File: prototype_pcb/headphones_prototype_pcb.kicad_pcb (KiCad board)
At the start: 2 copper layers, 59.8 x 62.2 mm, 52 parts, among them J1 LIGHTING_JACK, J2 CONN_01X10, J3 BOTTOM_FLEX_LIGHTNING, J4 CONN_01X10, J5 LIGHTNING_HEADPHONE_ADAPTER, J6 CONN_01X10, J7 IPHONE_HEADPHONE_JACK, J8 CONN_01X02, U1 SN74LVC1G123, U2 ADG774A, U3 SN74LVC1G123, U4 NC7S32

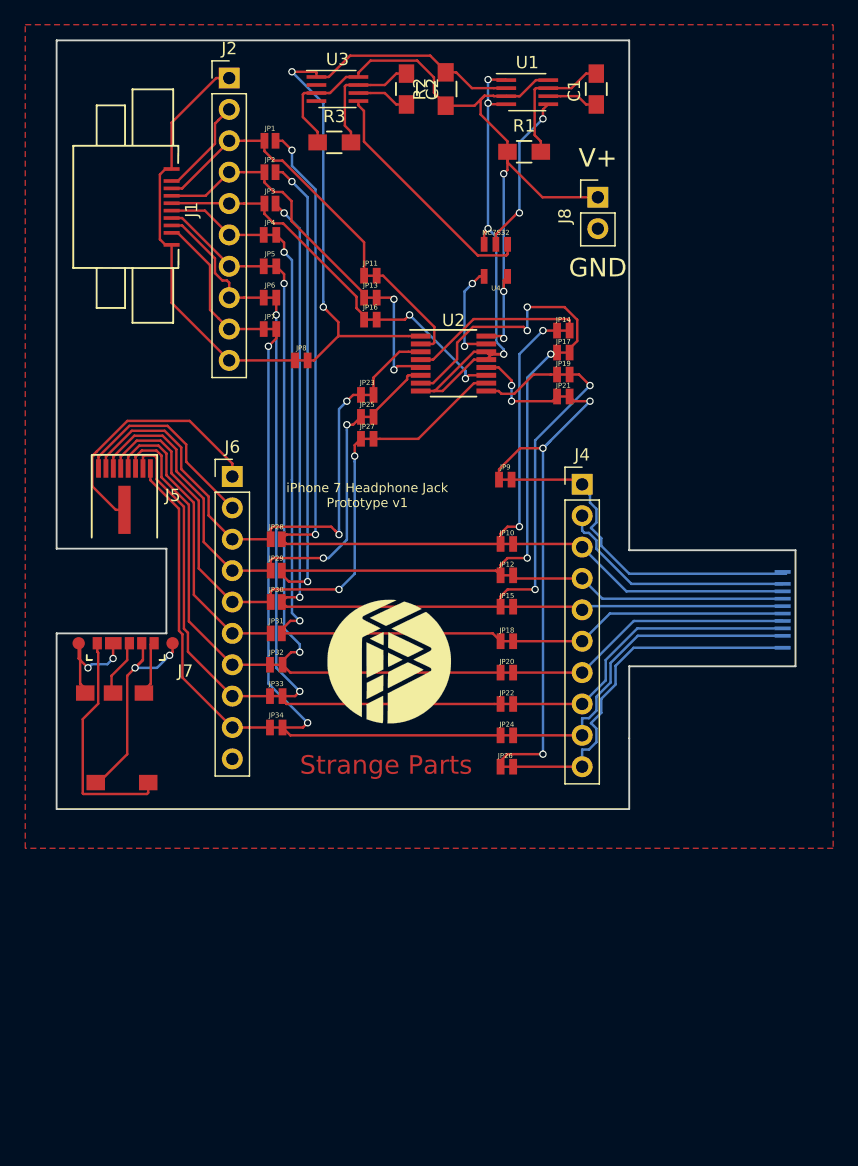
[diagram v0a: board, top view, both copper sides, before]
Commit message: Rigid prototype pcb v1.2
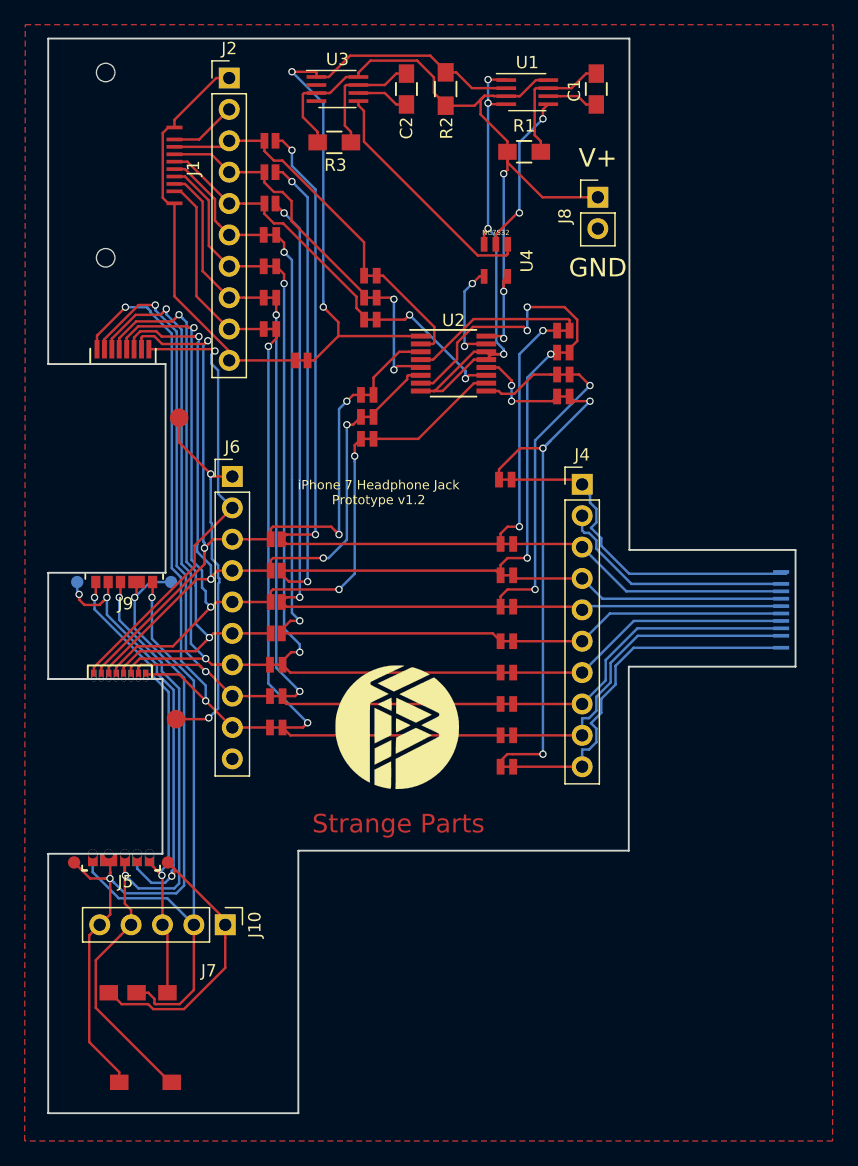
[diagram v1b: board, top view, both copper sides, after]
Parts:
- added J10: CONN_01X05, Pin_Headers:Pin_Header_Straight_1x05_Pitch2.54mm, F.Cu at (120.3, 128.8)
- added J9: LIGHTNING_HEADPHONE_ADAPTER, lightning_headphone_adapter:LIGHTNING_HEADPHONE_ADAPTER_HANDWIRE, F.Cu at (109.1, 83.3)
- J5: footprint lightning_headphone_adapter:LIGHTNING_HEADPHONE_ADAPTER -> lightning_headphone_adapter:LIGHTNING_HEADPHONE_ADAPTER_CASTELLATED
- moved J7 24.3 mm to (120.7, 142.4)
- moved J5 17.0 mm to (108.8, 107.8)
- moved G*** 5.35 mm to (134.2, 112.8)
- moved J1 3.37 mm to (112.5, 67.2)
- moved J3 0.13 mm to (162.1, 103.2)
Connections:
- J5 pad 11: Net-(J5-Pad11) -> Net-(J10-Pad2)
- J5 pad 12: Net-(J5-Pad12) -> Net-(J10-Pad5)
- J5 pad 13: Net-(J5-Pad13) -> Net-(J10-Pad4)
- J5 pad 14: Net-(J5-Pad14) -> Net-(J10-Pad1)
- J5 pad 16: Net-(J5-Pad12) -> Net-(J10-Pad5)
- J5 pad 17: Net-(J5-Pad14) -> Net-(J10-Pad1)
- J7 pad 1: Net-(J5-Pad12) -> Net-(J10-Pad1)
- J7 pad 2: Net-(J5-Pad13) -> Net-(J10-Pad2)
- J7 pad 4: Net-(J5-Pad11) -> Net-(J10-Pad4)
- J7 pad 5: Net-(J5-Pad14) -> Net-(J10-Pad5)
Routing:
- net Net-(J10-Pad5): track 0.00 -> 60.7 mm, vias 0 -> 2
- net Net-(J10-Pad1): track 0.00 -> 57.7 mm, vias 0 -> 3
- net Net-(J10-Pad4): track 0.00 -> 55.2 mm, vias 0 -> 2
- net Net-(J10-Pad2): track 0.00 -> 51.6 mm, vias 0 -> 1
- net Net-(J10-Pad3): track 4.51 -> 38.4 mm, vias 0 -> 2
- net Net-(J5-Pad9): track 26.8 -> 51.8 mm, vias 0 -> 2
- net Net-(J5-Pad7): track 25.8 -> 49.4 mm, vias 0 -> 2
- net Net-(J5-Pad8): track 27.1 -> 49.8 mm, vias 0 -> 2
- net Net-(J5-Pad6): track 24.6 -> 47.3 mm, vias 0 -> 2
- net /HPIN2: track 40.0 -> 62.3 mm, vias 2 -> 4
- net /HPIN4: track 42.7 -> 64.8 mm, vias 2 -> 4
- net /HPIN3: track 40.7 -> 62.5 mm, vias 2 -> 4
- net Net-(J5-Pad11): track 18.9 -> 0.00 mm
- net Net-(J5-Pad14): track 18.9 -> 0.00 mm, vias 2 -> 0
- net GNDREF: track 86.3 -> 104.3 mm, vias 4 -> 5
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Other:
- board size 59.8 x 62.2 mm -> 60.5 x 87 mm
- board text added: "iPhone 7 Headphone Jack Prototype v1.2"
- board text removed: "iPhone 7 Headphone Jack Prototype v1"
